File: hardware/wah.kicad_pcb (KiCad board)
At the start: 4 copper layers, 99.1 x 54.5 mm, 32 parts, among them J1 Barrel_Jack_Switch, J2 In, J3 Out, SW1 SW_Push_3PDT, U1 TL072, U2 L78L05_TO92

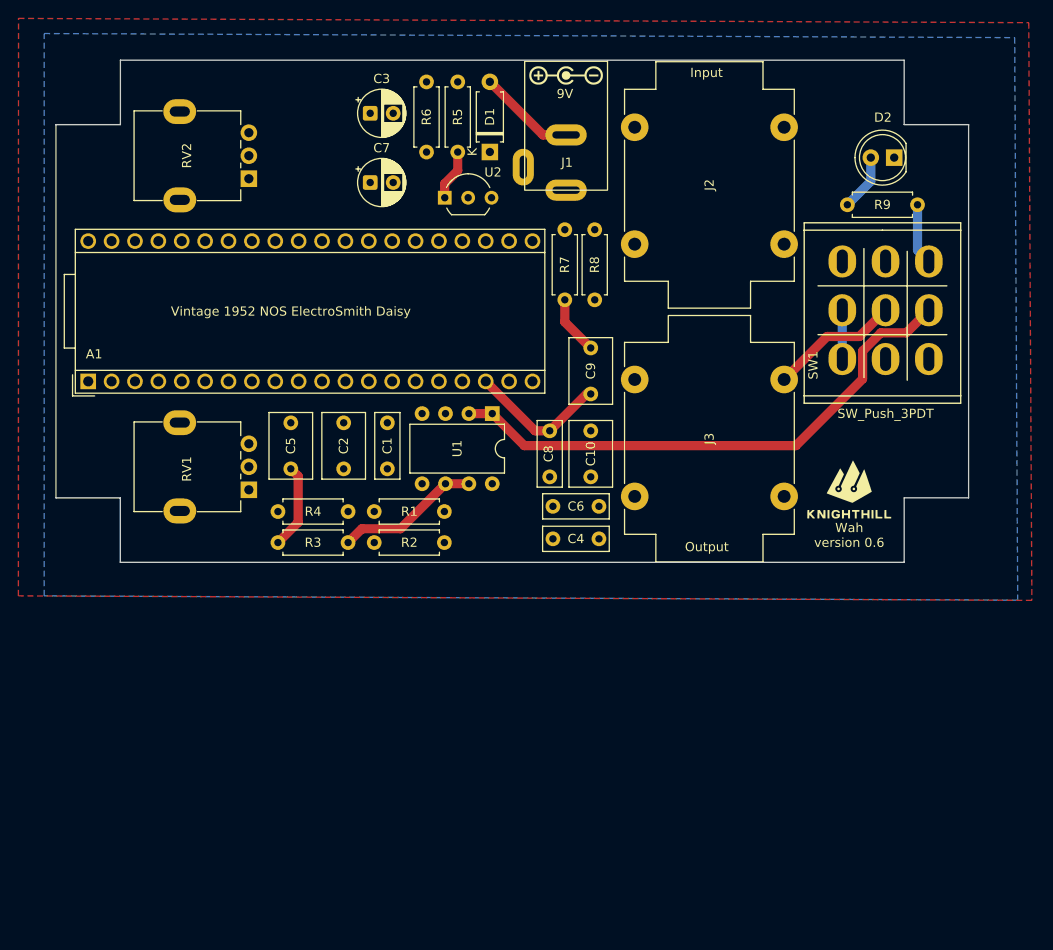
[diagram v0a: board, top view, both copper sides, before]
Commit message: pcb
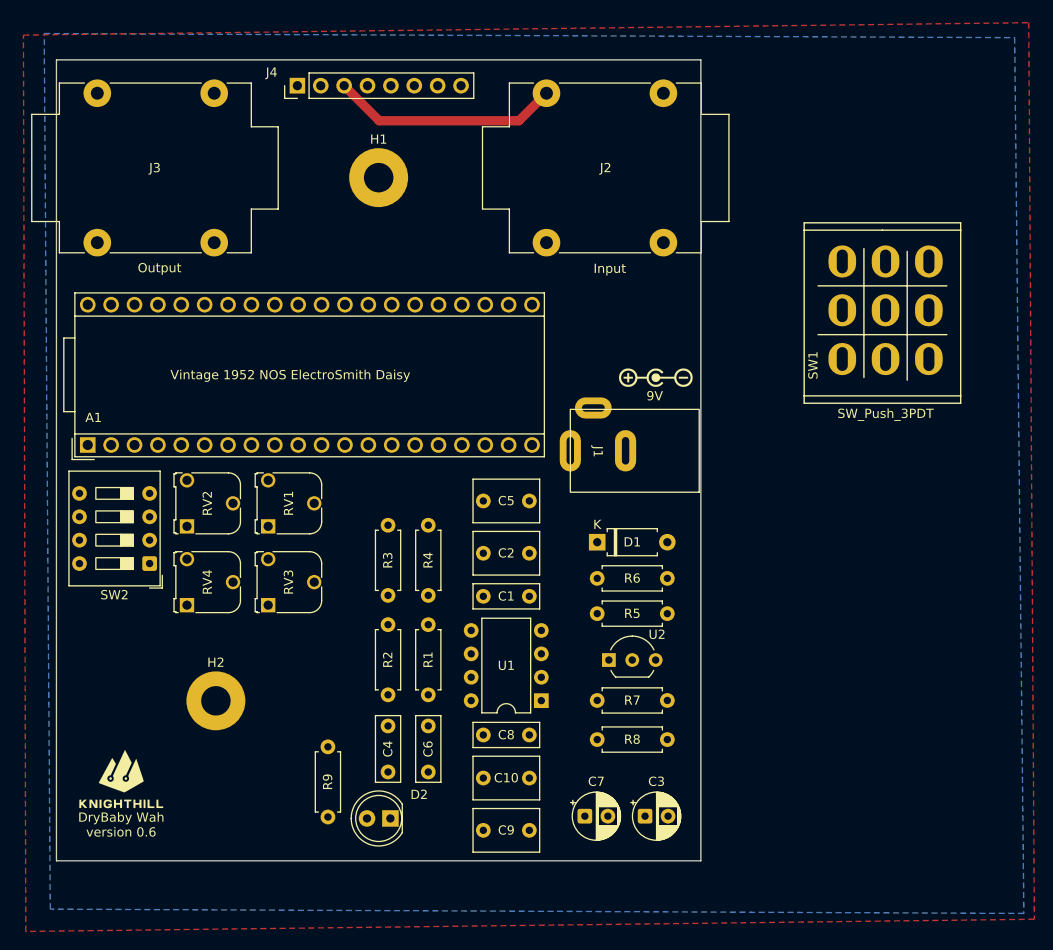
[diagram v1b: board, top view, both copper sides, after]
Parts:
- added H1: MountingHole_Pad, MountingHole:MountingHole_3.2mm_M3_Pad, F.Cu at (77.5, 45.9)
- added H2: MountingHole_Pad, MountingHole:MountingHole_3.2mm_M3_Pad, F.Cu at (59.8, 102.8)
- added J4: Conn_01x08_Pin, Connector_PinHeader_2.54mm:PinHeader_1x08_P2.54mm_Vertical, F.Cu at (68.6, 36.0)
- added RV3: 10k, Potentiometer_THT:Potentiometer_Runtron_RM-065_Vertical, F.Cu at (65.5, 92.4)
- added RV4: 10k, Potentiometer_THT:Potentiometer_Runtron_RM-065_Vertical, F.Cu at (56.6, 92.4)
- added SW2: SW_DIP_x04, Button_Switch_THT:SW_DIP_SPSTx04_Slide_9.78x12.34mm_W7.62mm_P2.54mm, F.Cu at (52.6, 87.9)
- RV1, RV2: footprint CustomFootprints:Potentiometer_uxcel_9mm_Single_Vertical -> Potentiometer_THT:Potentiometer_Runtron_RM-065_Vertical
- moved D2 90.3 mm to (78.7, 115.6)
- moved R9 87.0 mm to (72.0, 107.8), turned to -90 degrees
- moved G*** 85.1 mm to (49.4, 112.2)
- moved C3 82.0 mm to (106.4, 115.3)
- moved C7 72.7 mm to (99.9, 115.3)
- moved J3 63.7 mm to (59.6, 53.0), turned to 180 degrees
- moved R8 55.9 mm to (108.8, 107.0), turned to 180 degrees
- moved U2 53.3 mm to (102.5, 98.3)
- moved R5 52.4 mm to (101.2, 93.3), turned to 0 degrees
- moved R6 49.9 mm to (101.2, 89.5), turned to 0 degrees
- moved C9 48.8 mm to (88.8, 116.8), turned to 0 degrees
- moved R7 44.9 mm to (108.8, 102.7), turned to 180 degrees
- moved D1 44.0 mm to (101.2, 85.5), turned to 0 degrees
- moved RV2 38.4 mm to (56.6, 83.8), turned to 90 degrees
- moved C10 38.3 mm to (93.8, 111.2), turned to 180 degrees
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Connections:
- net Net-(J2-PadT) renamed /J_IN
- net Net-(J3-PadT) renamed /J_OUT
- A1 pad 22: unconnected-(A1-ADC_0-Pad22) -> /POT1
- A1 pad 24: /POT1 -> /POT3
- A1 pad 25: unconnected-(A1-ADC_3-Pad25) -> /POT4
- A1 pad 27: unconnected-(A1-ADC_5-Pad27) -> /SW1
- A1 pad 28: unconnected-(A1-ADC_6-Pad28) -> /SW2
- A1 pad 29: unconnected-(A1-DAC_OUT2-Pad29) -> /SW3
- A1 pad 30: unconnected-(A1-DAC_OUT1-Pad30) -> /SW4
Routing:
- net Net-(U1C-V+): track 58.9 -> 0.00 mm
- net Net-(U1A-+): track 42.1 -> 0.00 mm
- net /POT1: track 36.7 -> 0.00 mm
- net /POT2: track 29.6 -> 0.00 mm
- net /AUDIO_IN: track 28.8 -> 0.00 mm
- net /FX_OUT: track 59.3 -> 82.4 mm
- net /FX_IN: track 60.3 -> 78.5 mm
- net Net-(U1B-+): track 17.7 -> 0.00 mm
- net Net-(U1B--): track 15.8 -> 0.00 mm
- net /AUDIO_OUT: track 15.3 -> 0.00 mm
- net Net-(C1-Pad1): track 12.2 -> 0.00 mm
- net Net-(D1-A): track 10.7 -> 0.00 mm
- net /J_OUT: track 14.1 -> 23.9 mm
- net Net-(C5-Pad1): track 9.25 -> 0.00 mm
- net /J_IN: track 32.4 -> 24.8 mm
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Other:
- board size 99.1 x 54.5 mm -> 70 x 87 mm
- board text added: "DryBaby Wah version 0.6"
- board text removed: "Wah version 0.6"
